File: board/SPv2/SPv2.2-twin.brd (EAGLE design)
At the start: 56.5 x 22.9 mm, 38 parts, among them IC1 S34ML0XG1, IC2 F5508, IC4 74LS14DB, Q1 12MHz

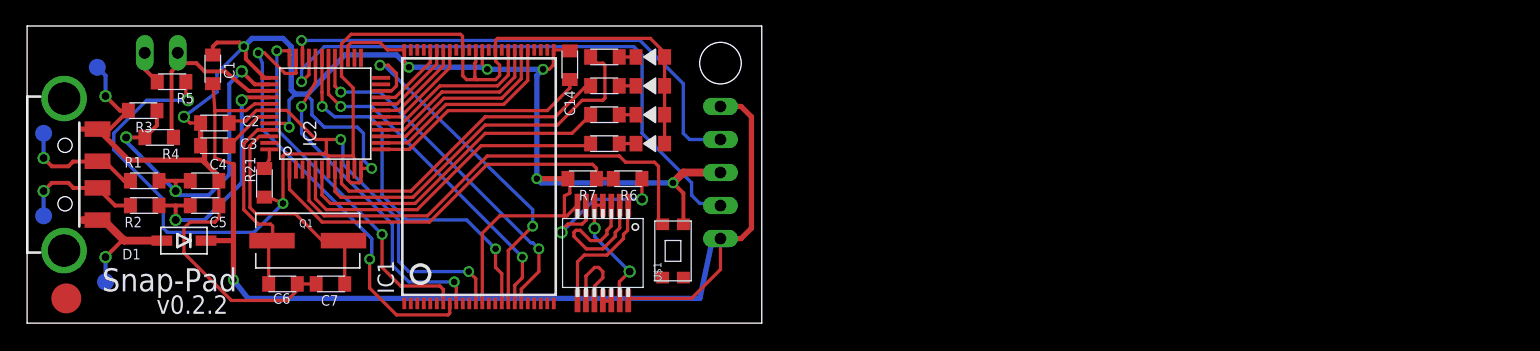
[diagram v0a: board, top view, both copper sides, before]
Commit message: finished v2.2, twinned board for fab
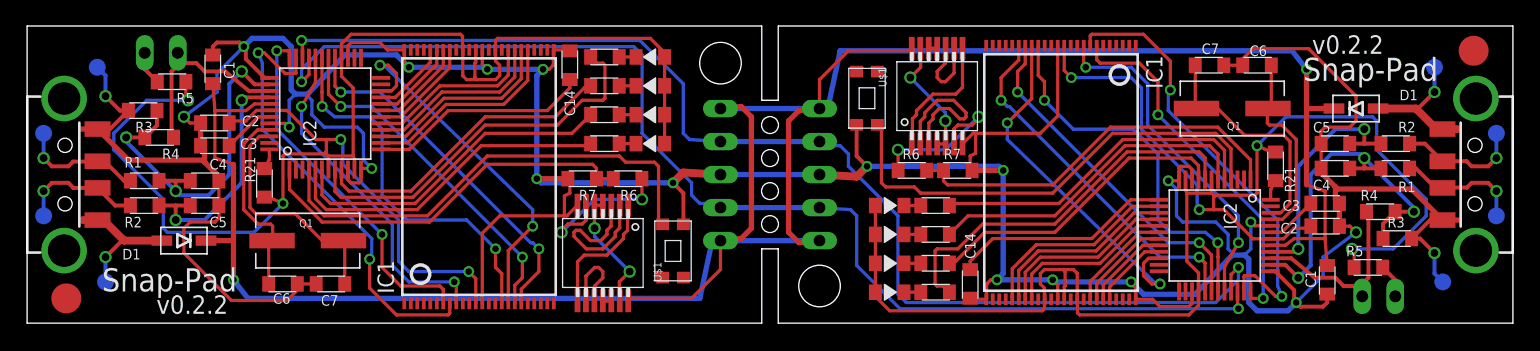
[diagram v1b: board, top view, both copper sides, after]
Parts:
- added C10, C9: 220nF, Passives:R0805
- added C11, C12, C13, C15: 20pF, Passives:R0805
- added C16, C8: 470nF, Passives:R0805
- added D2: (no value), Passives:SOD123
- added IC3: S34ML0XG1, Flash:TSOP48
- added IC5: F5508, TI_MSP430_v16:PT48
- added IC6: 74LS14DB, 74xx-db-us:SSOP14
- added JP2: USBA-SMD-MALE, Passives:USB-A-SMT-MALE
- added Q2: 12MHz, Passives:CSM-3X
- added R12, R13: 27 5%, Passives:R0805
- added R14, R17: 1M, Passives:R0805
- added R15: 1.4K 1%, Passives:R0805
- added R16, R18, R19, R20, R22: 130, Passives:R0805
- added R23, R24: 1.4k, Passives:R0805
- added SJ2: (no value), jumper:JP1
- added TP5, TP6, TP7, TP8: TPTP13R, testpad:TP13R
- added U$10, U$11, U$12, U$9: LED, Passives:LED0805
- added U$13: SNAP-HALF, Passives:SNAP-HALF
- added U$14: FIDUCAL, Passives:FIDUCAL
- added U$4: KMR-2, Passives:KMR-2-SWITCH
- moved U$2 0.16 mm to (58.4, 11.4)
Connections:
- new net !CE!_A1: IC3.9, IC5.32
- new net !RE!_A1: IC3.8, IC5.35
- new net !RST_A!1: IC5.48, R17.P$1
- new net !WE!_A1: IC3.18, IC5.30
- new net !WP!_A1: IC3.19, IC5.29
- new net +1V8_A1: C10.P$1, IC5.43
- new net +3V3_A1: C9.P$1, IC3.12, IC3.34, IC3.37, IC3.39, IC5.11, IC5.28, IC5.42, IC5.7, R16.P$2, R17.P$2, U$10.ANODE, U$11.ANODE, U$12.ANODE, U$9.ANODE
- new net ALE_A1: IC3.17, IC5.22
- new net CLE_A1: IC3.16, IC5.31
- new net D+_A1: C11.P$1, IC5.38, R12.P$1, R14.P$2, R15.P$1
- new net D-_A1: C12.P$1, IC5.40, R13.P$1
- new net DOUT1: IC5.1, R23.P$1, R24.P$2
- new net N$11: JP2.D+1, R12.P$2, TP5.TP
- new net N$12: JP2.D-1, R13.P$2, TP6.TP
- new net N$13: C16.P$1, IC5.13
- new net N$14: R20.P$1, U$11.CATHODE
- new net N$15: R19.P$1, U$10.CATHODE
- new net N$16: R18.P$1, U$9.CATHODE
- new net N$17: R22.P$1, U$12.CATHODE
- new net N$18: IC5.9, R22.P$2
- new net N$20: IC5.8, R20.P$2
- new net N$21: IC5.6, R19.P$2
- new net N$29: IC5.5, R18.P$2
- new net N$30: R16.P$1, SJ2.2
- new net N$31: D2.ANODE, JP2.VBUS1, TP7.TP
- new net N$32: IC6.11, IC6.12
- new net N$34: IC6.10, IC6.9
- new net N$35: IC6.1, IC6.8
- new net N$36: IC6.2, IC6.3
- new net N$37: IC6.13, IC6.4, IC6.5
- new net N$38: IC6.6, R23.P$2
- new net NANDIO_A10: IC3.31, IC5.16
- new net NANDIO_A11: IC3.32, IC5.17
- new net NANDIO_A12: IC3.41, IC5.18
- new net NANDIO_A13: IC3.42, IC5.19
- new net NANDIO_A14: IC3.43, IC5.20
- new net NANDIO_A15: IC3.44, IC5.21
- new net NANDIO_A8: IC3.29, IC5.14
- new net NANDIO_A9: IC3.30, IC5.15
- new net PUR_A1: IC5.39, R15.P$2, SJ2.1
- new net R/B_A1: IC3.7, IC5.36
- new net SW_A1: IC5.4, U$4.PB1, U$4.PB2
- new net TCK_A1: IC5.26
- new net TDI_A1: IC5.24
- new net TDO_A1: IC5.23
- new net TMS_A1: IC5.25
- new net TST_A1: IC5.47
- new net XT2IN_A1: C13.P$2, IC5.45, Q2.P$1
- new net XT2OUT_A1: C15.P$2, IC5.46, Q2.P$2
- net GND: now also C10.P$2, C11.P$2, C12.P$2, C13.P$1, C15.P$1, C16.P$2, C8.P$2, C9.P$2, IC3.13, IC3.25, IC3.36, IC3.48, IC5.10, IC5.12, IC5.27, IC5.37, IC5.44, IC6.7, JP2.GND1, R14.P$1, R24.P$1, TP8.TP, U$13.P$3, U$4.PA1, U$4.PA2
- net RX_A: now also IC5.33, U$13.P$2
- net TX_A: now also IC5.34, U$13.P$4
- net VBUS: now also C8.P$1, D2.CATHODE, IC5.41, IC6.14, U$13.P$1, U$13.P$5
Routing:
- net GND: track 163.6 -> 334.8 mm, vias 10 -> 20
- net +3V3_A1: track 0.00 -> 121.5 mm, vias 0 -> 4
- net VBUS: track 88.8 -> 192.6 mm, vias 1 -> 2
- net RX_A: track 39.0 -> 91.9 mm, vias 1 -> 2
- net TX_A: track 45.1 -> 91.9 mm, vias 1 -> 2
- net SW_A1: track 0.00 -> 36.6 mm
- net !RE!_A1: track 0.00 -> 34.3 mm, vias 0 -> 2
- net DOUT1: track 0.00 -> 30.3 mm
- net N$20: track 0.00 -> 29.7 mm
- net CLE_A1: track 0.00 -> 28.9 mm, vias 0 -> 2
- net D+_A1: track 0.00 -> 28.6 mm, vias 0 -> 3
- net ALE_A1: track 0.00 -> 28.1 mm, vias 0 -> 2
- net R/B_A1: track 0.00 -> 28.0 mm, vias 0 -> 2
- net !WP!_A1: track 0.00 -> 27.8 mm, vias 0 -> 2
- net !WE!_A1: track 0.00 -> 26.7 mm, vias 0 -> 2
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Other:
- board size 56.5 x 22.9 mm -> 114.3 x 22.9 mm
- board text added: "C1"
- board text added: "C14"
- board text added: "C2"
- board text added: "C3"
- board text added: "C4"
- board text added: "C5"
- board text added: "C6"
- board text added: "C7"
- board text added: "D1"
- board text added: "IC1"
- board text added: "IC2"
- board text added: "Q1"
- board text added: "R1"
- board text added: "R2"
- board text added: "R21"
- board text added: "R3"
- board text added: "R4"
- board text added: "R5"
- board text added: "R6"
- board text added: "R7"
- board text added: "TP1"
- board text added: "TP2"
- board text added: "TP3"
- board text added: "TP4"
- board text added: "U$1"
